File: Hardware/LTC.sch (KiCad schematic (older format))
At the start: 64 parts, among them J10 Conn_01x01_Female, J11 Conn_01x01_Female, J12 Conn_01x01_Female, J6 Conn_01x01_Female, J7 Conn_01x01_Female, J8 Conn_01x01_Female, J9 Conn_01x01_Female, Q2 Q_PMOS_GSD, Q3 Q_PMOS_GSD, Q4 Q_PMOS_GSD, Q5 Q_PMOS_GSD, Q6 Q_PMOS_GSD, Q7 Q_PMOS_GSD, Q8 Q_PMOS_GSD, Q9 Q_NPN_BCE

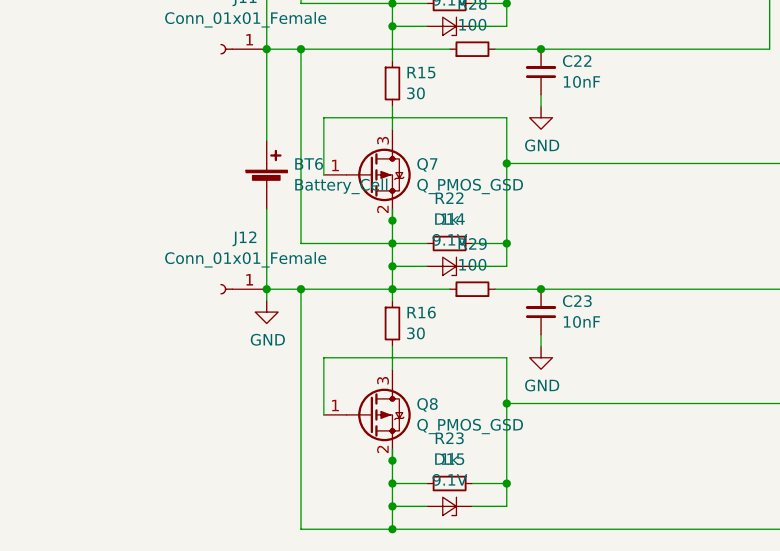
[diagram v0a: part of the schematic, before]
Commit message: ZCO version
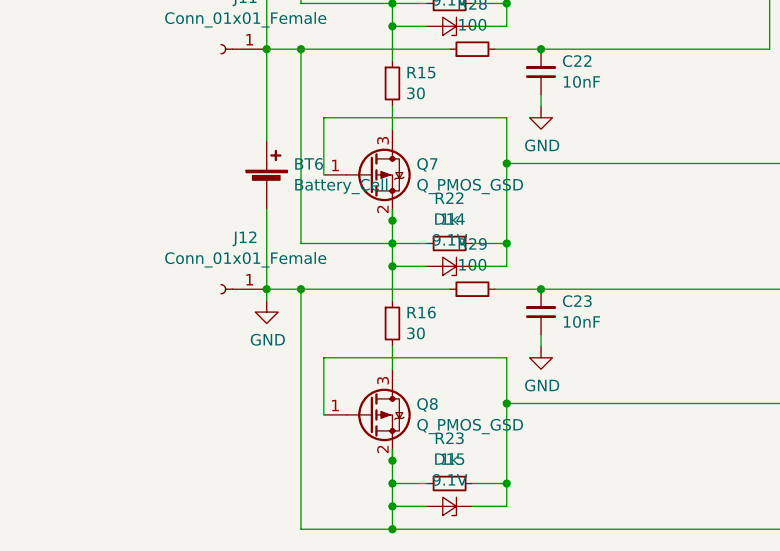
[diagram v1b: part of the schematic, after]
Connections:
- net GND: no longer BT5.2 (-), BT6.1 (+), D14.2 (A), J11.1 (Pin_1), Q7.2 (S), R16.1, R22.2, R28.1
- new net: BT5.2 (-), BT6.1 (+), D14.2 (A), J11.1 (Pin_1), Q7.2 (S), R16.1, R22.2, R28.1
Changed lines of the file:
@@
 Wire Wire Line
 	5350 8550 5350 3450
-Wire Wire Line
-	3600 8550 3850 8550
-Wire Wire Line
-	3600 8550 3600 8600
-Connection ~ 3600 8550
 Connection ~ 3600 9600
 Wire Wire Line
@@
 	4100 9050 4100 8850
 Connection ~ 4100 9050
-Wire Wire Line
-	3200 8550 3600 8550
-Connection ~ 3200 8550
 Wire Wire Line
 	3050 8550 3200 8550
@@
 	4250 6450 5150 6450
 Wire Wire Line
-	5150 3050 5150 6450
-Wire Wire Line
 	4100 5900 5100 5900
 Wire Wire Line
-	5100 2950 5100 5900
-Wire Wire Line
 	4250 5400 5050 5400
 Wire Wire Line
-	5050 5400 5050 2850
-Wire Wire Line
-	4100 4850 5000 4850
-Wire Wire Line
 	5000 4850 5000 2750
 Wire Wire Line
-	4250 4350 4950 4350
-Wire Wire Line
 	4950 4350 4950 2650
-Wire Wire Line
-	4100 3800 4900 3800
 Wire Wire Line
 	4900 3800 4900 2550
@@
 	3050 8550 3050 8200
 Connection ~ 3600 8450
-Wire Wire Line
-	3600 8450 3600 8550
 Wire Wire Line
 	4100 8000 4100 8350
@@
 Connection ~ 3600 5300
 Wire Wire Line
-	4100 4850 4100 5200
-Wire Wire Line
-	4100 4850 4100 4650
-Connection ~ 4100 4850
-Wire Wire Line
 	3200 4350 3850 4350
 Connection ~ 3200 4350
@@
 Wire Wire Line
 	3600 5050 3600 5100
-$Comp
-L power:GND #PWR037
-U 1 1 600FD82C
-P 4250 4600
-F 0 "#PWR037" H 4250 4350 50  0001 C CNN
-F 1 "GND" H 4255 4427 50  0000 C CNN
-F 2 "" H 4250 4600 50  0001 C CNN
-F 3 "" H 4250 4600 50  0001 C CNN
-	1    4250 4600
-	1    0    0    -1
-$EndComp
 Wire Wire Line
 	4250 4550 4250 4600
 Wire Wire Line
 	3050 4350 3050 4750
-Connection ~ 4250 4350
 $Comp
 L Device:R_Small R25
@@
 	4050 4350 4250 4350
 $Comp
-L Device:C_Small C19
-U 1 1 600FD81B
-P 4250 4450
-F 0 "C19" H 4158 4404 50  0000 R CNN
-F 1 "10nF" H 4158 4495 50  0000 R CNN
-F 2 "Capacitor_SMD:C_1206_3216Metric" H 4250 4450 50  0001 C CNN
-F 3 "~" H 4250 4450 50  0001 C CNN
-	1    4250 4450
-	-1   0    0    1
-$EndComp
-$Comp
 L Device:Battery_Cell BT3
 U 1 1 600FD815
@@
 	3050 4350 3050 4000
 Connection ~ 3600 4250
-Wire Wire Line
-	4100 3800 4100 4150
-Wire Wire Line
-	4100 3800 4100 3600
-Connection ~ 4100 3800
 Wire Wire Line
 	4100 2750 4100 3100
@@
 Wire Wire Line
 	3600 4000 3600 4050
-$Comp
-L power:GND #PWR036
-U 1 1 5FFC24FD
-P 4250 3550
-F 0 "#PWR036" H 4250 3300 50  0001 C CNN
-F 1 "GND" H 4255 3377 50  0000 C CNN
-F 2 "" H 4250 3550 50  0001 C CNN
-F 3 "" H 4250 3550 50  0001 C CNN
-	1    4250 3550
-	1    0    0    -1
-$EndComp
 Wire Wire Line
 	4250 3500 4250 3550
@@
 Wire Wire Line
 	6450 1500 6450 1650
+Connection ~ 4100 3800
+Wire Wire Line
+	4100 3800 4100 3600
+Wire Wire Line
+	4100 3800 4100 4150
+Connection ~ 4250 4350
+Connection ~ 4100 4850
+Wire Wire Line
+	4100 4850 4100 4650
+Wire Wire Line
+	4100 4850 4100 5200
+Wire Wire Line
+	5150 3050 5150 6450
+Wire Wire Line
+	5100 2950 5100 5900
+Wire Wire Line
+	5050 5400 5050 2850
+$Comp
+L power:GND #PWR036
+U 1 1 5FFC24FD
+P 4250 3550
+F 0 "#PWR036" H 4250 3300 50  0001 C CNN
+F 1 "GND" H 4255 3377 50  0000 C CNN
+F 2 "" H 4250 3550 50  0001 C CNN
+F 3 "" H 4250 3550 50  0001 C CNN
+	1    4250 3550
+	1    0    0    -1
+$EndComp
+$Comp
+L Device:C_Small C19
+U 1 1 600FD81B
+P 4250 4450
+F 0 "C19" H 4158 4404 50  0000 R CNN
+F 1 "10nF" H 4158 4495 50  0000 R CNN
+F 2 "Capacitor_SMD:C_1206_3216Metric" H 4250 4450 50  0001 C CNN
+F 3 "~" H 4250 4450 50  0001 C CNN
+	1    4250 4450
+	-1   0    0    1
+$EndComp
+$Comp
+L power:GND #PWR037
+U 1 1 600FD82C
+P 4250 4600
+F 0 "#PWR037" H 4250 4350 50  0001 C CNN
+F 1 "GND" H 4255 4427 50  0000 C CNN
+F 2 "" H 4250 4600 50  0001 C CNN
+F 3 "" H 4250 4600 50  0001 C CNN
+	1    4250 4600
+	1    0    0    -1
+$EndComp
+Wire Wire Line
+	4100 3800 4900 3800
+Wire Wire Line
+	4250 4350 4950 4350
+Wire Wire Line
+	4100 4850 5000 4850
+Wire Wire Line
+	3600 8450 3600 8600
+Wire Wire Line
+	3200 8550 3850 8550
+Connection ~ 3200 8550
 $EndSCHEMATC

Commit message: Going back to work
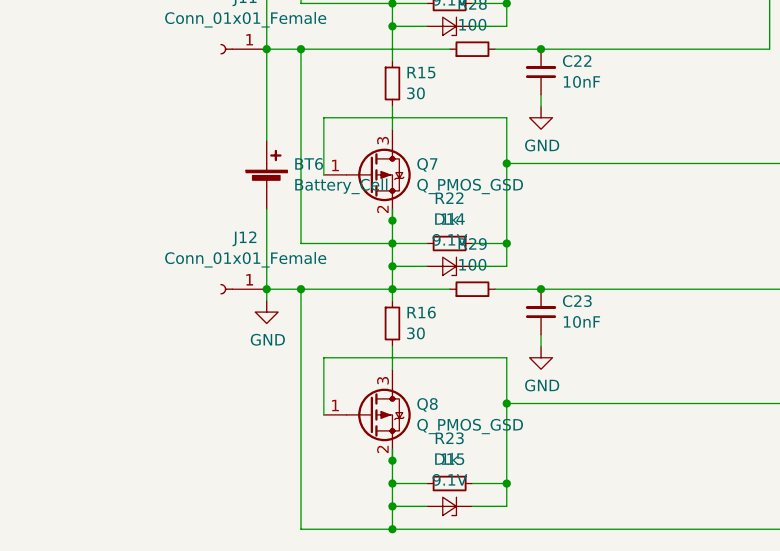
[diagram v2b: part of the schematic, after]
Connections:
- net GND: now also BT5.2 (-), BT6.1 (+), D14.2 (A), J11.1 (Pin_1), Q7.2 (S), R16.1, R22.2, R28.1
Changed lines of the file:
@@
 Wire Wire Line
 	5350 8550 5350 3450
+Wire Wire Line
+	3600 8550 3850 8550
+Wire Wire Line
+	3600 8550 3600 8600
+Connection ~ 3600 8550
 Connection ~ 3600 9600
 Wire Wire Line
@@
 	4100 9050 4100 8850
 Connection ~ 4100 9050
+Wire Wire Line
+	3200 8550 3600 8550
+Connection ~ 3200 8550
 Wire Wire Line
 	3050 8550 3200 8550
@@
 	4250 6450 5150 6450
 Wire Wire Line
+	5150 3050 5150 6450
+Wire Wire Line
 	4100 5900 5100 5900
 Wire Wire Line
+	5100 2950 5100 5900
+Wire Wire Line
 	4250 5400 5050 5400
 Wire Wire Line
+	5050 5400 5050 2850
+Wire Wire Line
+	4100 4850 5000 4850
+Wire Wire Line
 	5000 4850 5000 2750
 Wire Wire Line
+	4250 4350 4950 4350
+Wire Wire Line
 	4950 4350 4950 2650
+Wire Wire Line
+	4100 3800 4900 3800
 Wire Wire Line
 	4900 3800 4900 2550
@@
 	3050 8550 3050 8200
 Connection ~ 3600 8450
+Wire Wire Line
+	3600 8450 3600 8550
 Wire Wire Line
 	4100 8000 4100 8350
@@
 Connection ~ 3600 5300
 Wire Wire Line
+	4100 4850 4100 5200
+Wire Wire Line
+	4100 4850 4100 4650
+Connection ~ 4100 4850
+Wire Wire Line
 	3200 4350 3850 4350
 Connection ~ 3200 4350
@@
 Wire Wire Line
 	3600 5050 3600 5100
+$Comp
+L power:GND #PWR037
+U 1 1 600FD82C
+P 4250 4600
+F 0 "#PWR037" H 4250 4350 50  0001 C CNN
+F 1 "GND" H 4255 4427 50  0000 C CNN
+F 2 "" H 4250 4600 50  0001 C CNN
+F 3 "" H 4250 4600 50  0001 C CNN
+	1    4250 4600
+	1    0    0    -1
+$EndComp
 Wire Wire Line
 	4250 4550 4250 4600
 Wire Wire Line
 	3050 4350 3050 4750
+Connection ~ 4250 4350
 $Comp
 L Device:R_Small R25
@@
 	4050 4350 4250 4350
 $Comp
+L Device:C_Small C19
+U 1 1 600FD81B
+P 4250 4450
+F 0 "C19" H 4158 4404 50  0000 R CNN
+F 1 "10nF" H 4158 4495 50  0000 R CNN
+F 2 "Capacitor_SMD:C_1206_3216Metric" H 4250 4450 50  0001 C CNN
+F 3 "~" H 4250 4450 50  0001 C CNN
+	1    4250 4450
+	-1   0    0    1
+$EndComp
+$Comp
 L Device:Battery_Cell BT3
 U 1 1 600FD815
@@
 	3050 4350 3050 4000
 Connection ~ 3600 4250
+Wire Wire Line
+	4100 3800 4100 4150
+Wire Wire Line
+	4100 3800 4100 3600
+Connection ~ 4100 3800
 Wire Wire Line
 	4100 2750 4100 3100
@@
 Wire Wire Line
 	3600 4000 3600 4050
+$Comp
+L power:GND #PWR036
+U 1 1 5FFC24FD
+P 4250 3550
+F 0 "#PWR036" H 4250 3300 50  0001 C CNN
+F 1 "GND" H 4255 3377 50  0000 C CNN
+F 2 "" H 4250 3550 50  0001 C CNN
+F 3 "" H 4250 3550 50  0001 C CNN
+	1    4250 3550
+	1    0    0    -1
+$EndComp
 Wire Wire Line
 	4250 3500 4250 3550
@@
 Wire Wire Line
 	6450 1500 6450 1650
-Connection ~ 4100 3800
-Wire Wire Line
-	4100 3800 4100 3600
-Wire Wire Line
-	4100 3800 4100 4150
-Connection ~ 4250 4350
-Connection ~ 4100 4850
-Wire Wire Line
-	4100 4850 4100 4650
-Wire Wire Line
-	4100 4850 4100 5200
-Wire Wire Line
-	5150 3050 5150 6450
-Wire Wire Line
-	5100 2950 5100 5900
-Wire Wire Line
-	5050 5400 5050 2850
-$Comp
-L power:GND #PWR036
-U 1 1 5FFC24FD
-P 4250 3550
-F 0 "#PWR036" H 4250 3300 50  0001 C CNN
-F 1 "GND" H 4255 3377 50  0000 C CNN
-F 2 "" H 4250 3550 50  0001 C CNN
-F 3 "" H 4250 3550 50  0001 C CNN
-	1    4250 3550
-	1    0    0    -1
-$EndComp
-$Comp
-L Device:C_Small C19
-U 1 1 600FD81B
-P 4250 4450
-F 0 "C19" H 4158 4404 50  0000 R CNN
-F 1 "10nF" H 4158 4495 50  0000 R CNN
-F 2 "Capacitor_SMD:C_1206_3216Metric" H 4250 4450 50  0001 C CNN
-F 3 "~" H 4250 4450 50  0001 C CNN
-	1    4250 4450
-	-1   0    0    1
-$EndComp
-$Comp
-L power:GND #PWR037
-U 1 1 600FD82C
-P 4250 4600
-F 0 "#PWR037" H 4250 4350 50  0001 C CNN
-F 1 "GND" H 4255 4427 50  0000 C CNN
-F 2 "" H 4250 4600 50  0001 C CNN
-F 3 "" H 4250 4600 50  0001 C CNN
-	1    4250 4600
-	1    0    0    -1
-$EndComp
-Wire Wire Line
-	4100 3800 4900 3800
-Wire Wire Line
-	4250 4350 4950 4350
-Wire Wire Line
-	4100 4850 5000 4850
-Wire Wire Line
-	3600 8450 3600 8600
-Wire Wire Line
-	3200 8550 3850 8550
-Connection ~ 3200 8550
 $EndSCHEMATC

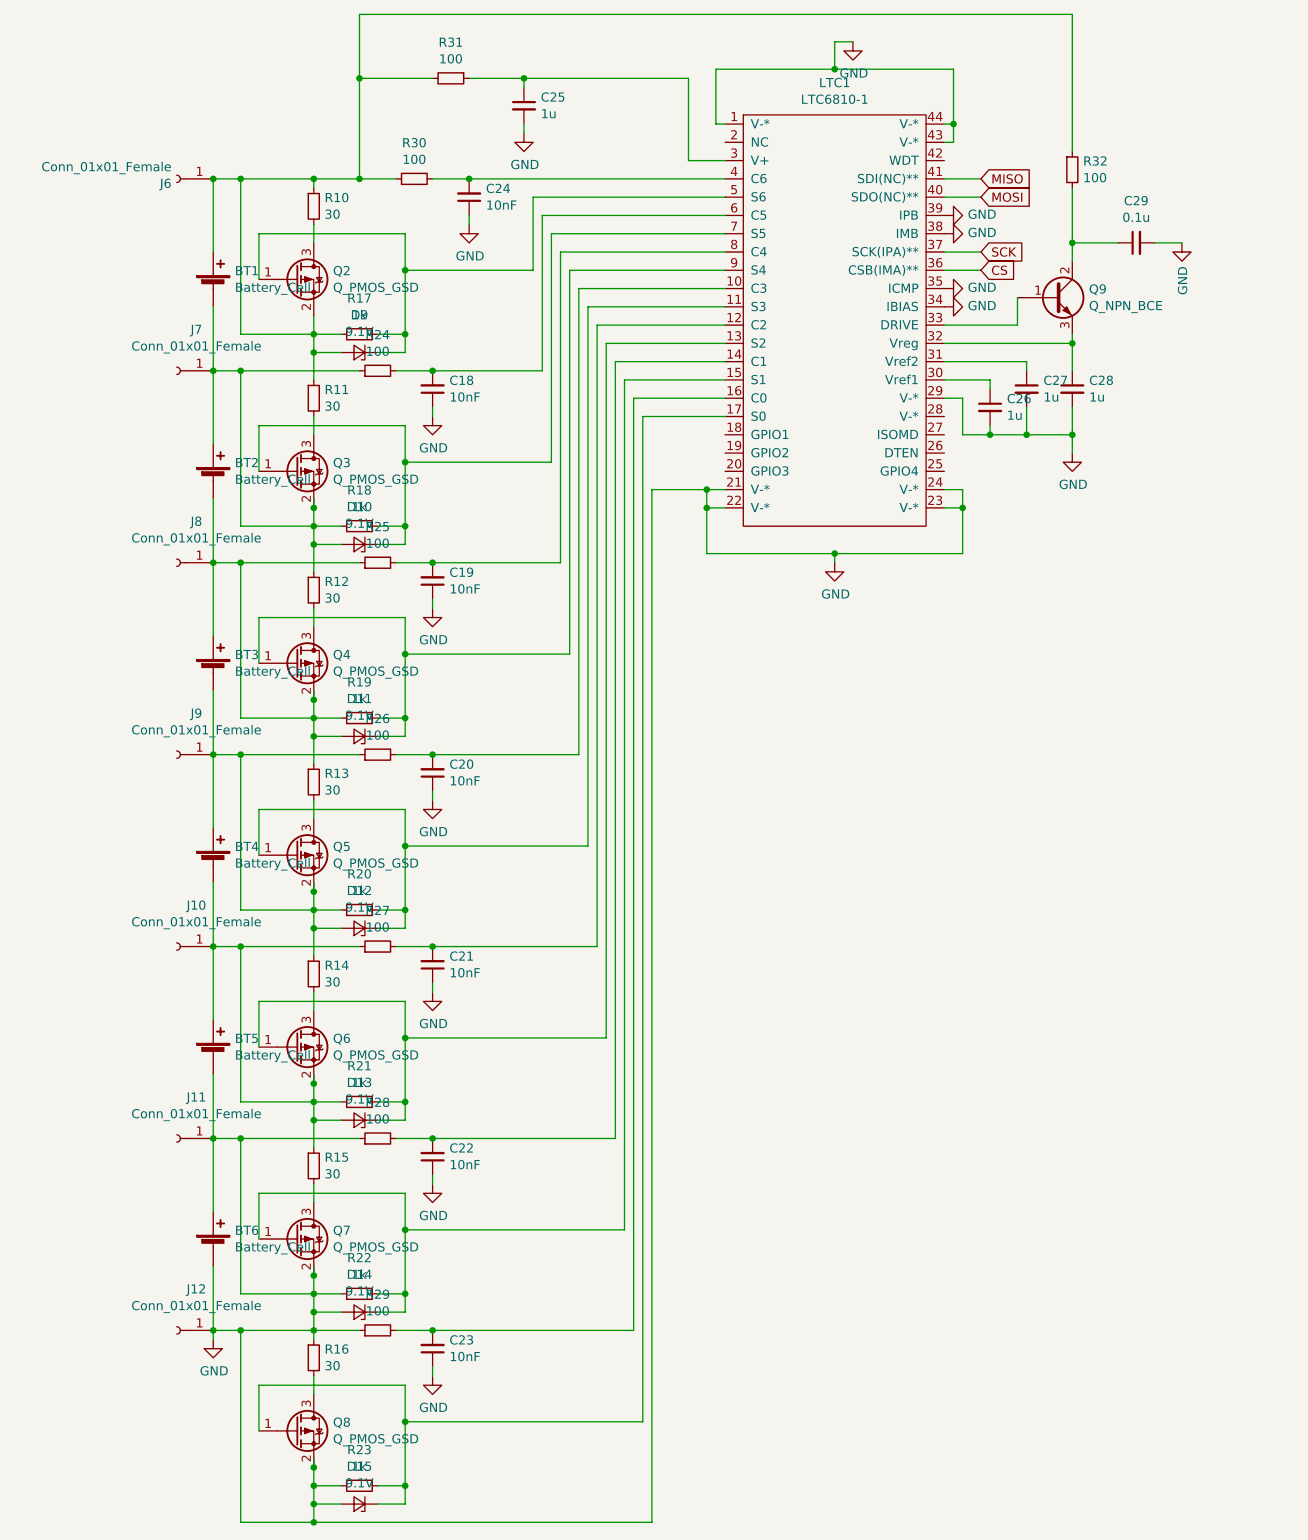
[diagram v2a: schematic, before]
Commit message: pcb layout nearly done
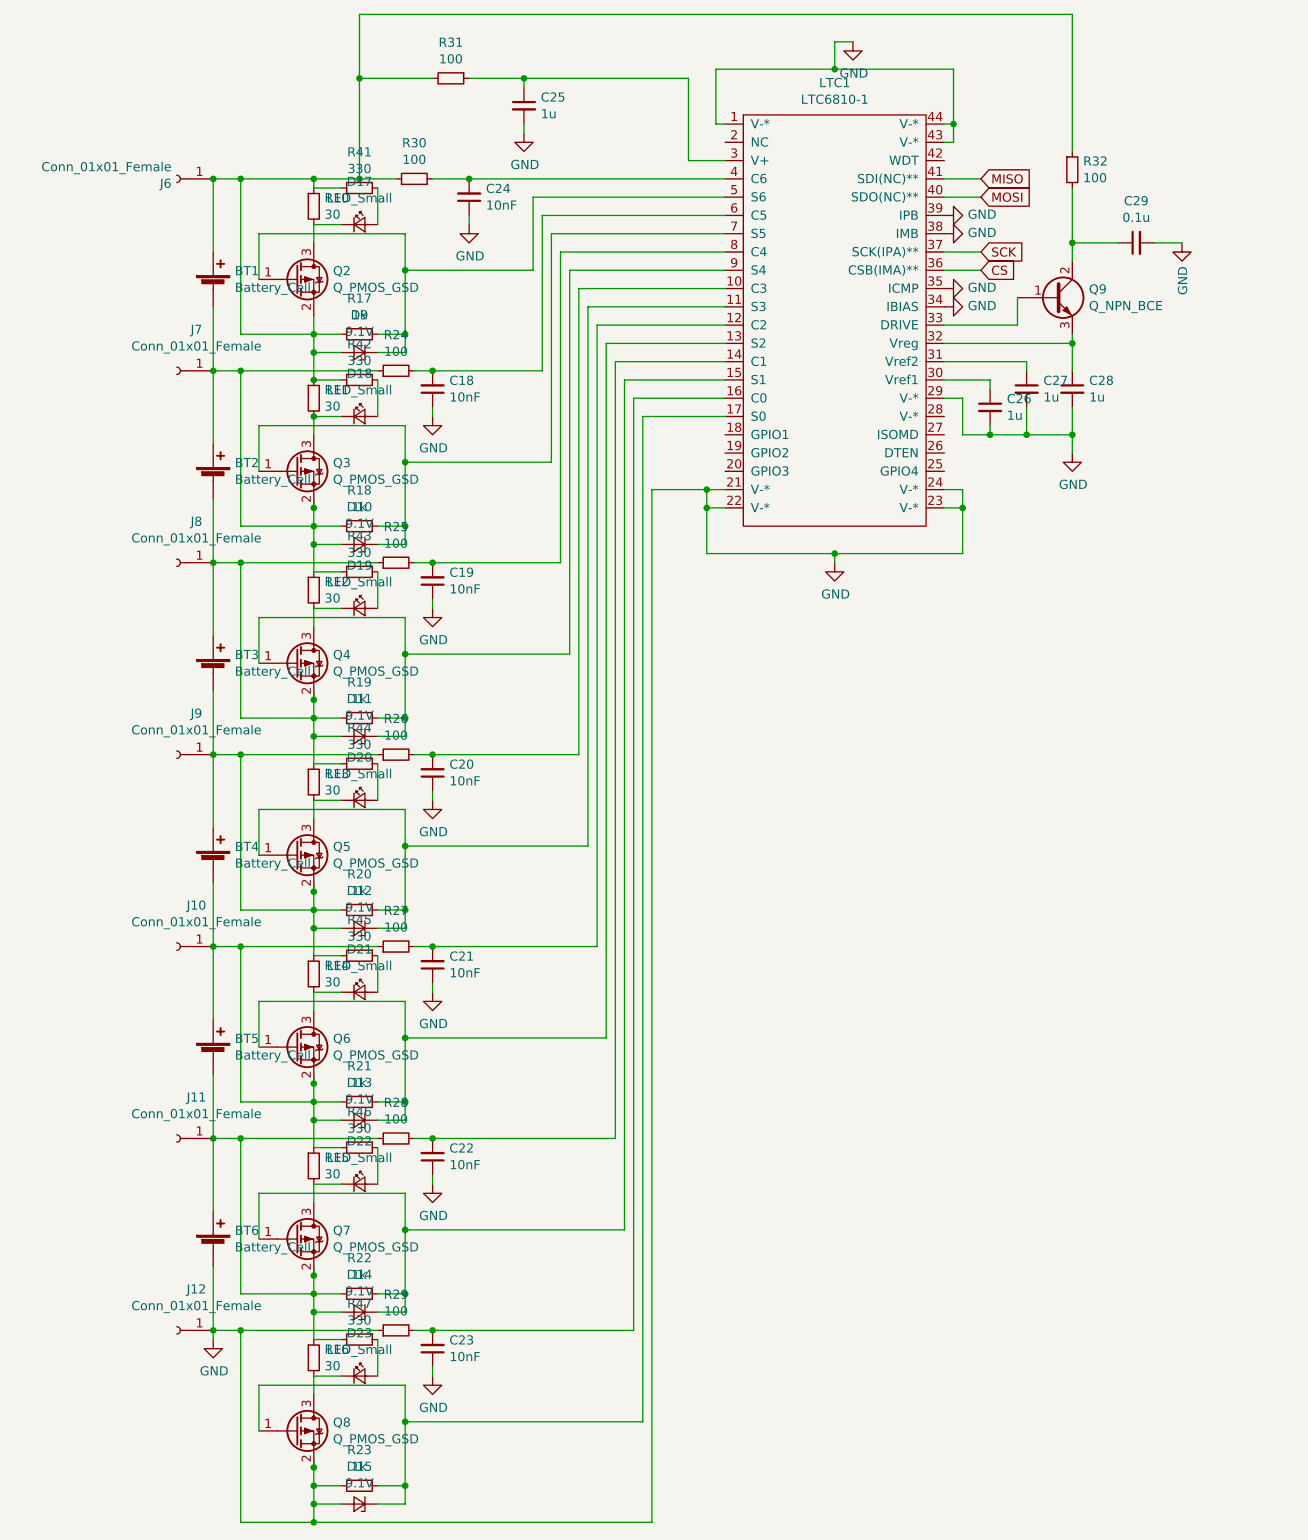
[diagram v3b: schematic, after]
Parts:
- added D17, D18, D19, D20, D21, D22, D23: LED_Small, LED_SMD:LED_0805_2012Metric, symbol Device:LED_Small
- added R41, R42, R43, R44, R45, R46, R47: 330, Resistor_SMD:R_1206_3216Metric, symbol Device:R_Small
- J10, J11, J12, J6, J7, J8, J9: footprint Connector_Pin:Pin_D1.0mm_L10.0mm_LooseFit -> CellPad:CellPad
- R10, R11, R12, R13, R14, R15, R16: footprint Resistor_SMD:R_1206_3216Metric -> Resistor_SMD:R_2512_6332Metric
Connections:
- net GND: no longer BT5.2 (-), BT6.1 (+), D14.2 (A), J11.1 (Pin_1), Q7.2 (S), R16.1, R22.2, R28.1
- net at BT1.1 (+), D9.2 (A), J6.1 (Pin_1)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: now also R41.2, R42.2
- net at Q2.3 (D), R10.2: now also D17.1 (K)
- net at BT1.2 (-), BT2.1 (+), D10.2 (A)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: now also R43.2
- net at Q3.3 (D), R11.2: now also D18.1 (K)
- net at BT2.2 (-), BT3.1 (+), D11.2 (A)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: now also R44.2
- net at BT3.2 (-), BT4.1 (+), D12.2 (A)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: now also R45.2
- net at Q4.3 (D), R12.2: now also D19.1 (K)
- net at BT4.2 (-), BT5.1 (+), D13.2 (A)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: now also R46.2
- net at Q5.3 (D), R13.2: now also D20.1 (K)
- net at Q6.3 (D), R14.2: now also D21.1 (K)
- net at Q7.3 (D), R15.2: now also D22.1 (K)
- net at Q8.3 (D), R16.2: now also D23.1 (K)
- new net: BT5.2 (-), BT6.1 (+), D14.2 (A), J11.1 (Pin_1), Q7.2 (S), R16.1, R22.2, R28.1, R47.2
- new net: D18.2 (A), R42.1
- new net: D17.2 (A), R41.1
- new net: D19.2 (A), R43.1
- new net: D20.2 (A), R44.1
- new net: D21.2 (A), R45.1
- new net: D22.2 (A), R46.1
- new net: D23.2 (A), R47.1
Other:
- moved on the sheet: R24, R25, R26, R27, R28, R29
